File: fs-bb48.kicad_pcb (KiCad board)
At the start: 2 copper layers, 35 x 12.1 mm, 15 parts, among them P1 USB, P2 SWD, P3 PWR, P4 EXT, T1 TOUCH_PAD, U1 MKL27Z256VFM4, U2 EMIF02-USB03F2

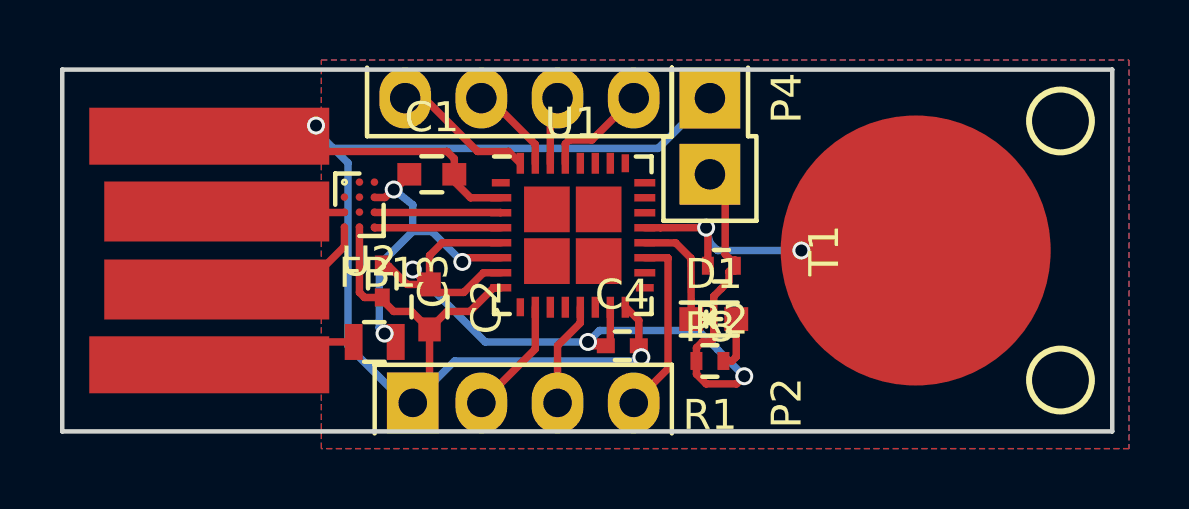
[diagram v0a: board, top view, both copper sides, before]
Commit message: update
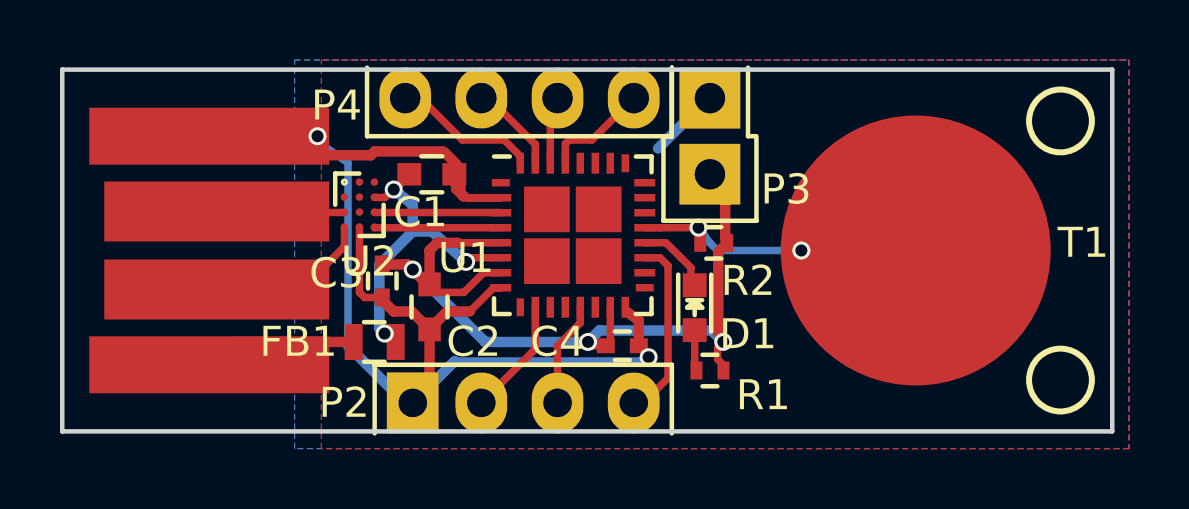
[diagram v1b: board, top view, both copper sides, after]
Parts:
- added FST-LOGO: VAL**, fs-bb48:FST-LOGO, B.Cu at (159.0, 106.7)
- added H1: 2mm, fs-bb48:Hole, F.Cu at (159.8, 102.6)
- FB1: value 330Ohm -> 330ohm
- moved R2 0.80 mm to (148.2, 106.7)
- moved D1 0.74 mm to (147.6, 108.8), turned to 270 degrees
- moved R1 0.32 mm to (148.1, 110.9), turned to 0 degrees
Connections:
- net Net-(C1-Pad1) renamed /VBUS
- net Net-(D1-Pad1) renamed /LED
- net Net-(FB1-Pad1) renamed /VBUS_
- net Net-(P1-Pad2) renamed /D-_
- net Net-(P1-Pad3) renamed /D+_
- net Net-(P2-Pad1) renamed /RESET
- net Net-(P2-Pad2) renamed /SWD_DIO
- net Net-(P2-Pad3) renamed /SWD_CLK
- net Net-(P4-Pad1) renamed /PTD4
- net Net-(P4-Pad2) renamed /PTD5
- net Net-(P4-Pad3) renamed /PTD6
- net Net-(P4-Pad4) renamed /PTD7
- net Net-(R2-Pad2) renamed /TOUCH
- net Net-(U1-Pad3) renamed /D+
- net Net-(U1-Pad4) renamed /D-
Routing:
- net GND: track 62.0 -> 56.4 mm
- net +3V3: track 36.8 -> 32.8 mm
- net /LED: track 3.78 -> 2.52 mm
- net /D+_: track 5.05 -> 4.08 mm
- net /TOUCH: track 10.8 -> 9.92 mm
- net /PTD7: track 5.50 -> 6.27 mm
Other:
- net class GND added: clearance 0.2, trace_width 0.7, via_dia 0.6, via_drill 0.4
- board text added: "FS-BB48"
- board text added: "Flying Stone Technology"
